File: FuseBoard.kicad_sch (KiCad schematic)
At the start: 22 parts, among them J1 Conn_01x02_Socket, J10 Conn_01x02_Socket, J2 Conn_01x02_Socket, J3 Conn_01x02_Socket, J4 Conn_01x02_Socket, J5 Conn_01x02_Socket, J6 Conn_01x02_Socket, J7 Conn_01x02_Socket, J8 Conn_01x02_Socket, J9 Conn_01x02_Socket

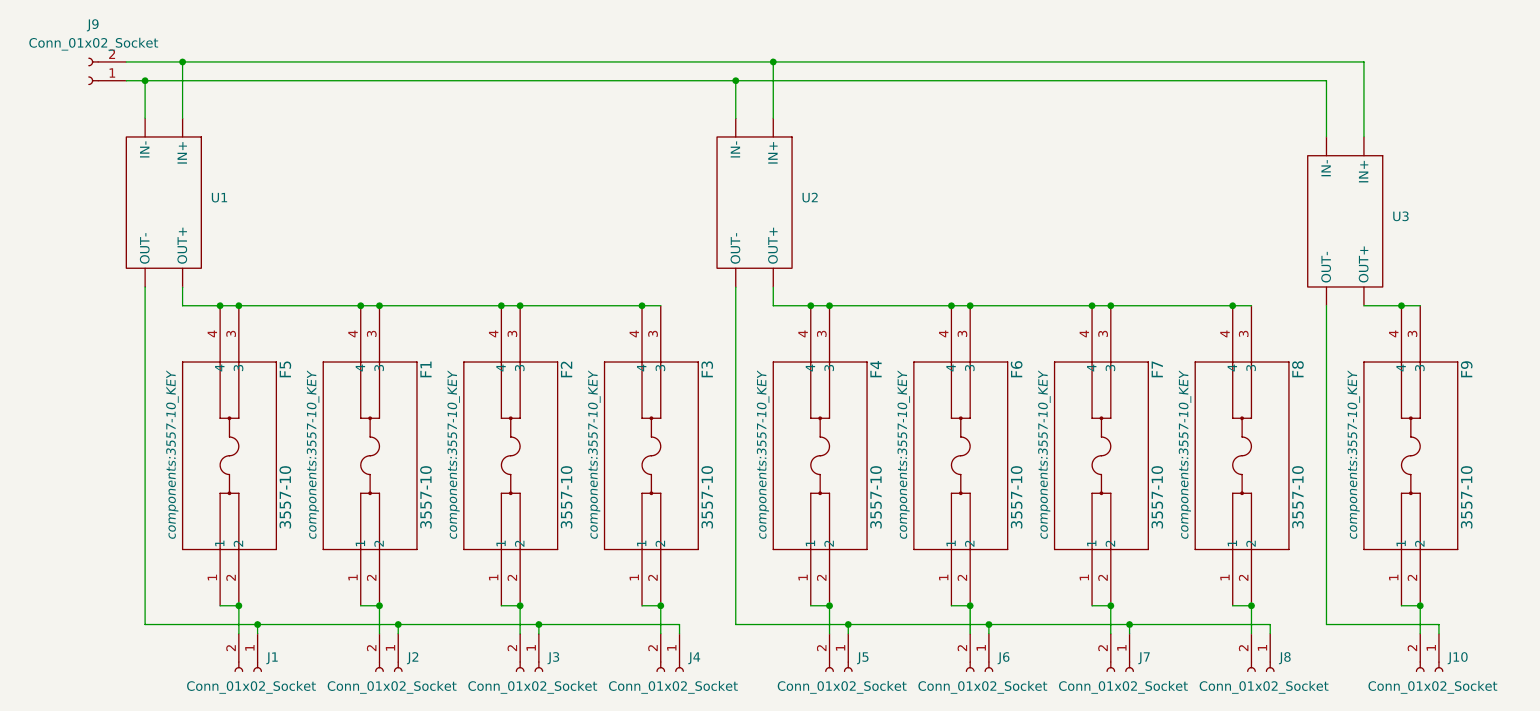
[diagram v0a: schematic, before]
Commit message: changes to pcb
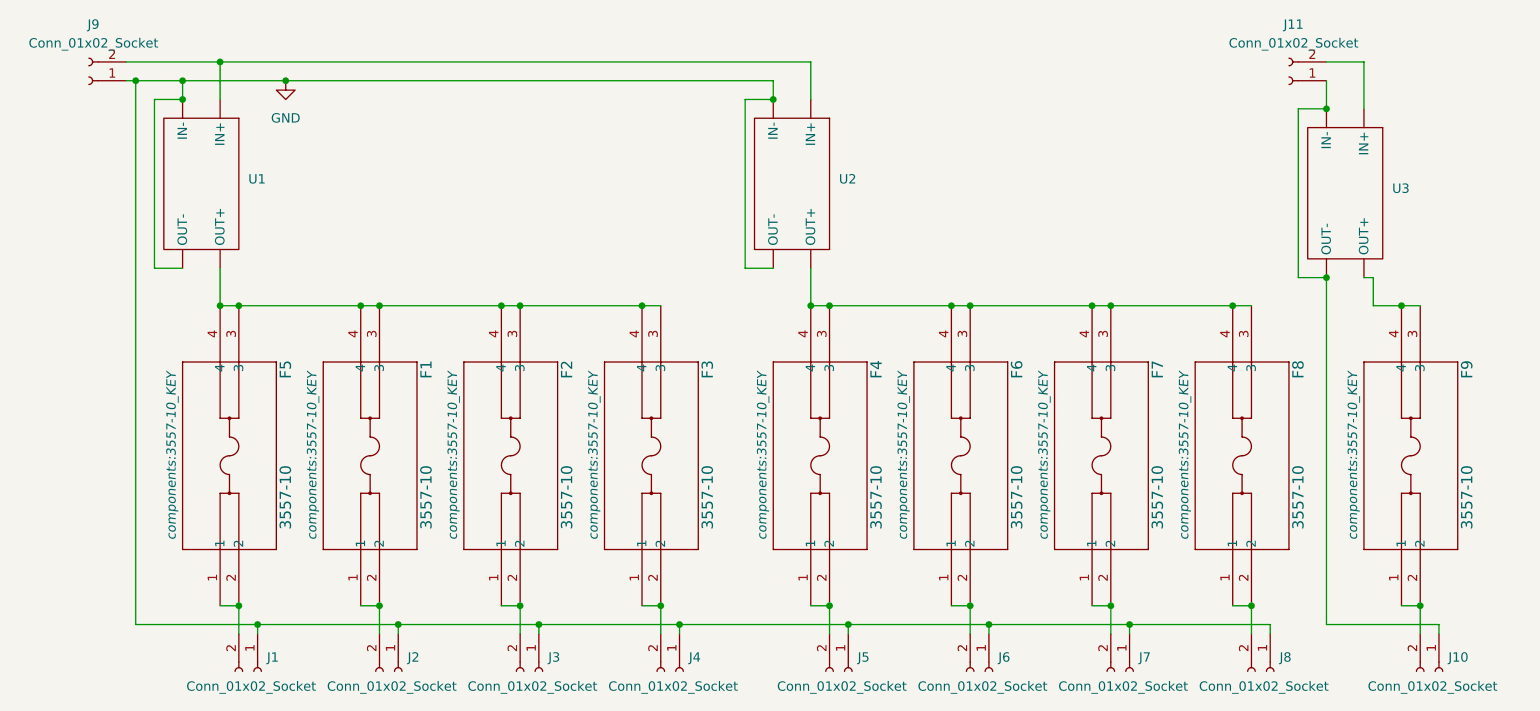
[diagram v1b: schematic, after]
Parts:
- added J11: Conn_01x02_Socket, Connector_AMASS:AMASS_XT30PW-M_1x02_P2.50mm_Horizontal, symbol Connector:Conn_01x02_Socket
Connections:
- net GND: now reaches J1.1 (Pin_1), J2.1 (Pin_1), J3.1 (Pin_1), J4.1 (Pin_1), U1. (OUT-)
- net GND: now also J5.1 (Pin_1), J6.1 (Pin_1), J7.1 (Pin_1), J8.1 (Pin_1), J9.1 (Pin_1), U2. (OUT-)
- net at J10.1 (Pin_1), U3. (OUT-): now also J11.1 (Pin_1)
- new net: J11.2 (Pin_2), U3. (OUT-)
- new net: J9.2 (Pin_2), U1. (OUT-), U2. (OUT-)
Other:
- moved on the sheet: U1, U2, U3
